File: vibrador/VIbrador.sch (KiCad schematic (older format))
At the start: 8 parts, among them U1 Pila3,7V, U2 StepDown, U3 Buzzer, U4 HC-05, U5 Buzzer, U6 PiZeroW, U7 Pila3,7V-Modulos-VIbrador-res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

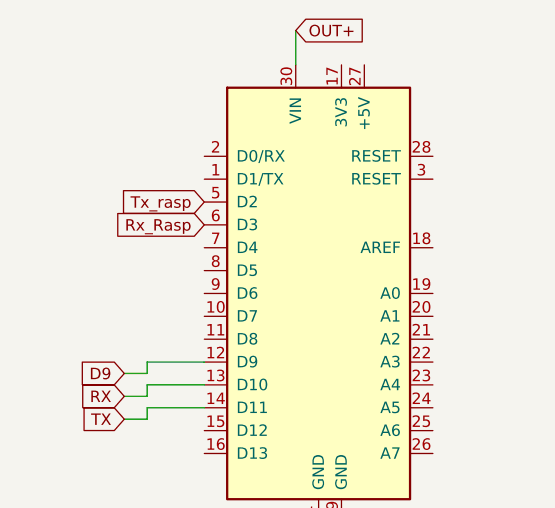
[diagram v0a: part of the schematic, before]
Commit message: Se guardo el  PCB finallizado
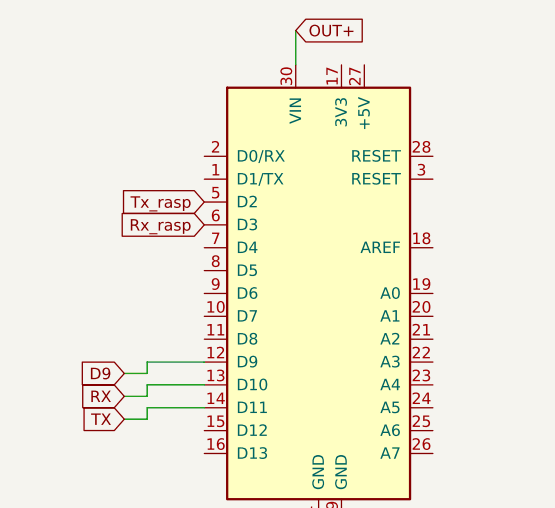
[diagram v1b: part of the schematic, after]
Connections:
- net Rx_Rasp is gone; now on net Rx_rasp: A1.6 (D3)
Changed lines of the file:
@@
 Tx_rasp
 Text GLabel 2350 2200 0    50   Input ~ 0
-Rx_Rasp
+Rx_rasp
 Text GLabel 3850 4650 2    50   Input ~ 0
 Tx_rasp
